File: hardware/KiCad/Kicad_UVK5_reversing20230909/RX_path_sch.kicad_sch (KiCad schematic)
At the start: 42 parts, among them J21 Conn_Coaxial, J22 Conn_Coaxial, J23 Conn_Coaxial, Q21 2SC3356, Q22 2SC3356

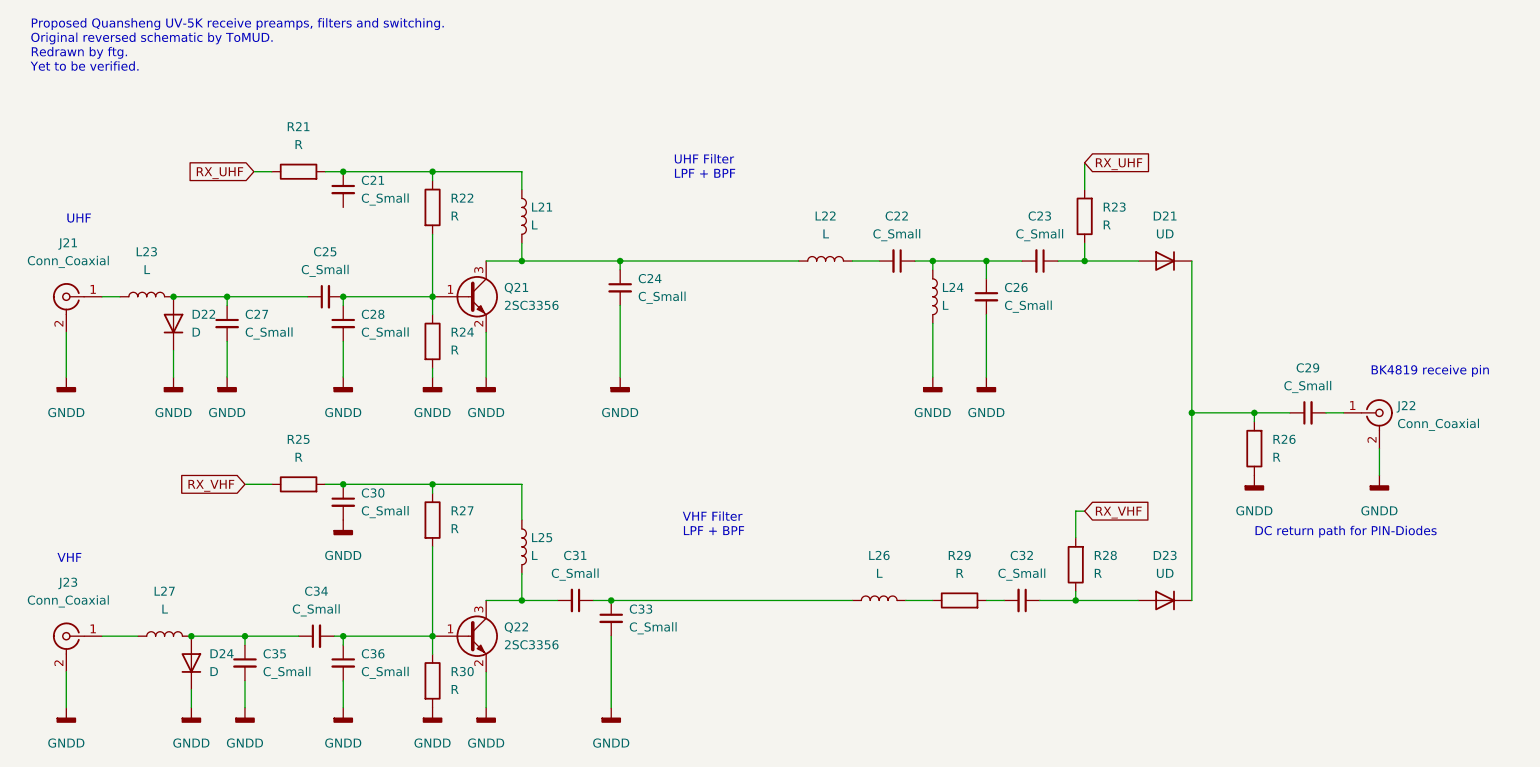
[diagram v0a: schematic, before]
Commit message: Add files via upload
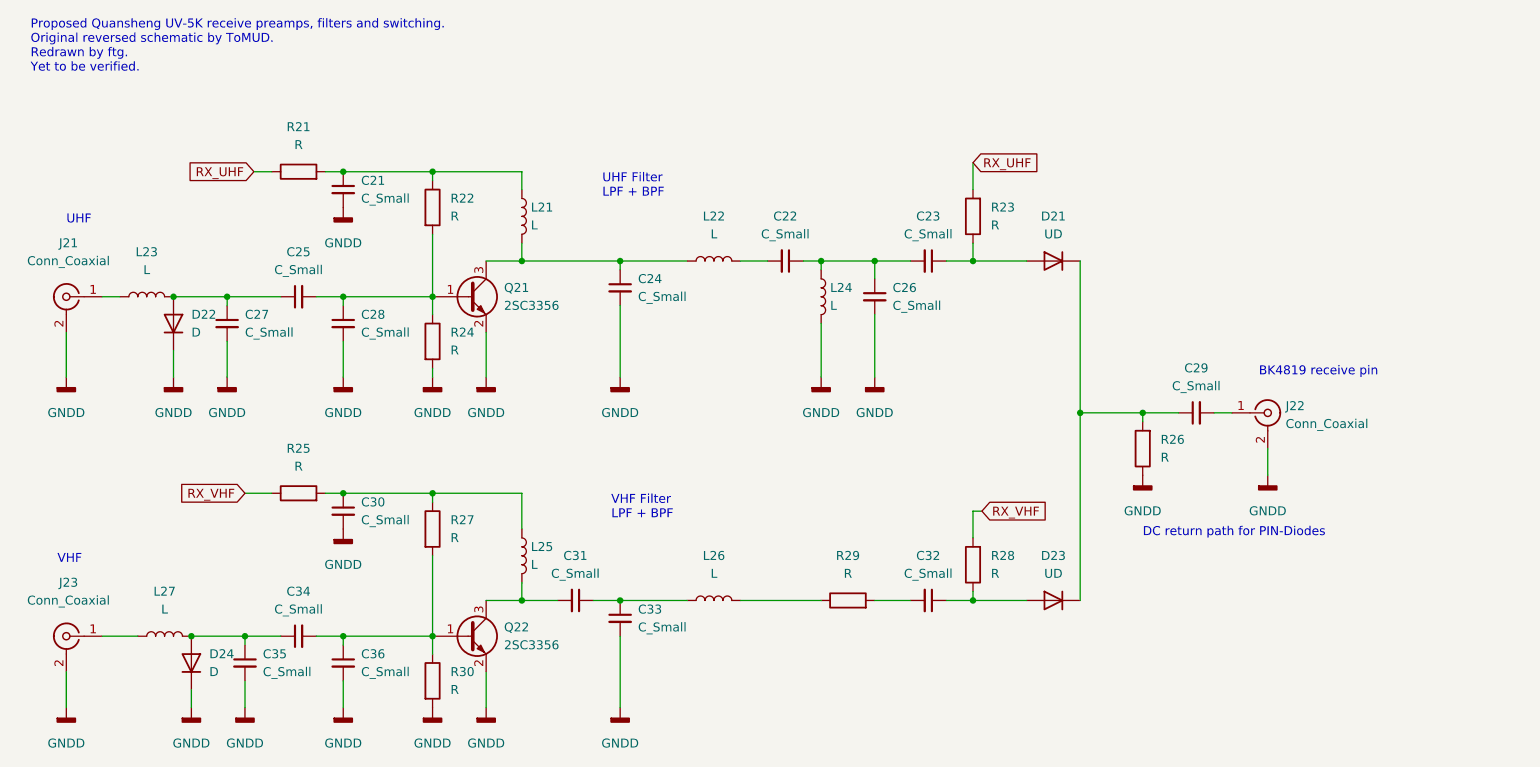
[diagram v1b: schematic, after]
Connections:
- net GNDD: now also C21.2
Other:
- moved on the sheet: C22, C23, C25, C26, C29, C30, C32, C33, C34, D21, D23, J22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
